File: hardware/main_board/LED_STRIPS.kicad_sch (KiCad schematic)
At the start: 9 parts, among them IC801 SN74AHCT125DBR, J801 Conn_01x03_Pin, J802 Conn_01x03_Pin

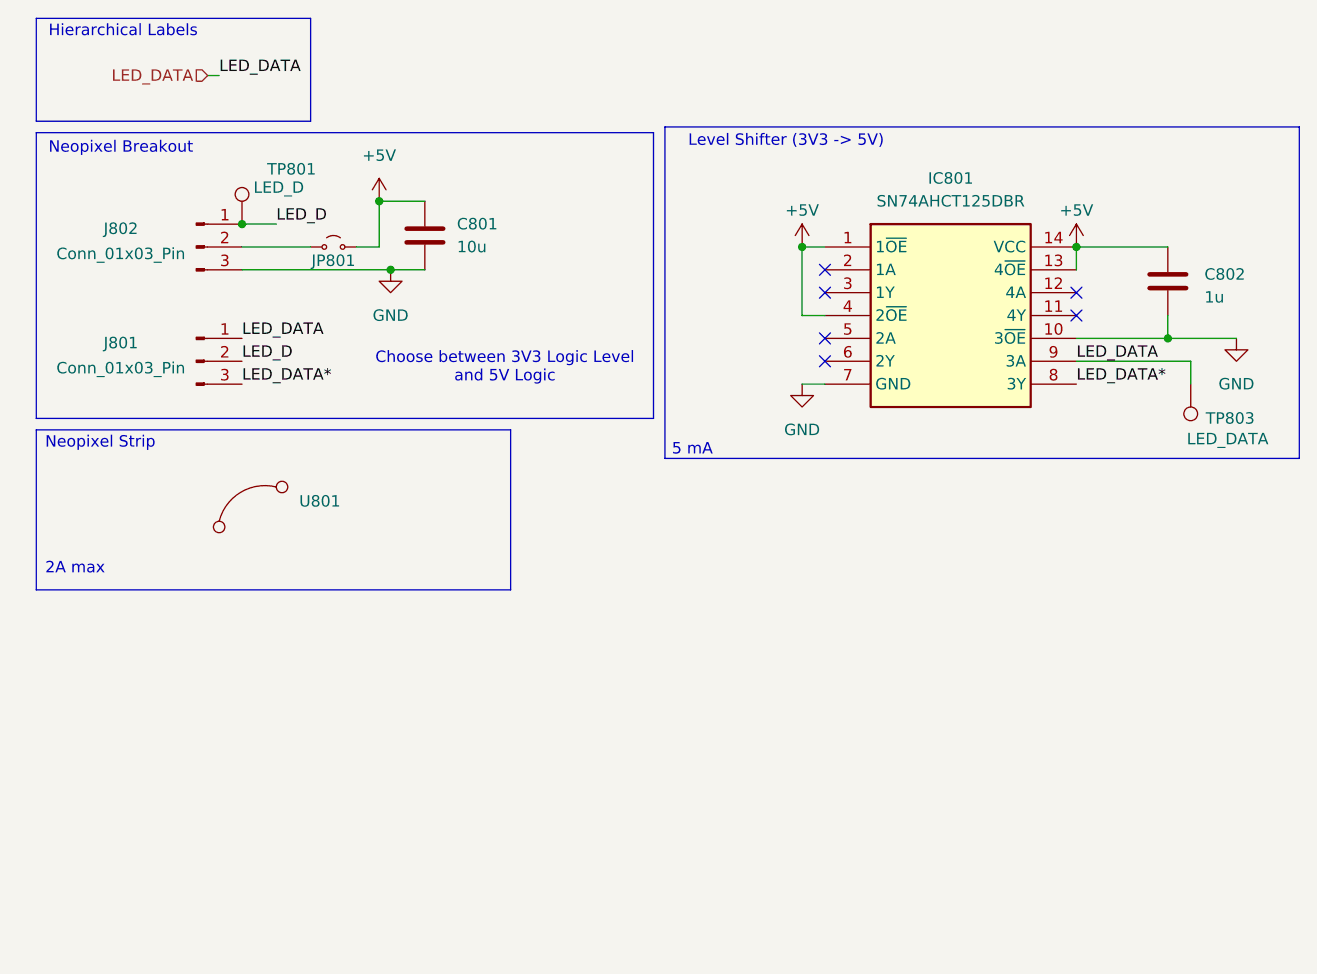
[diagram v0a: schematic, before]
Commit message: pcb review changes
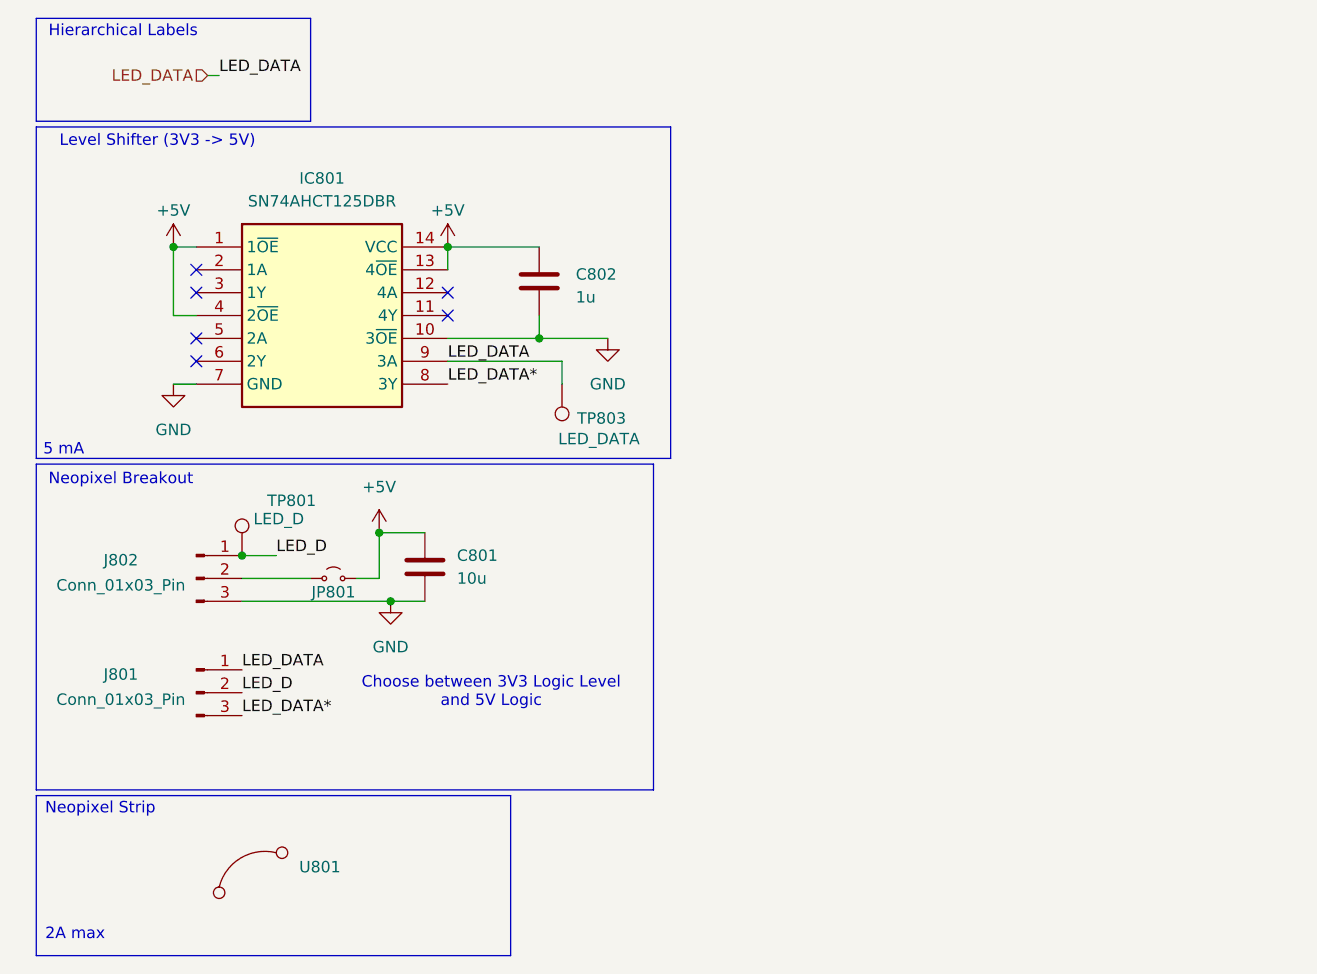
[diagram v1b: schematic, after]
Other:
- moved on the sheet: C801, C802, IC801, J801, J802, JP801, TP801, TP803, U801
